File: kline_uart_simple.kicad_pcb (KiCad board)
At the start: 4 copper layers, 9 parts, among them J1 USB2UART, J2 KLINE_CONN, Q1 BC547, Q2 BC547

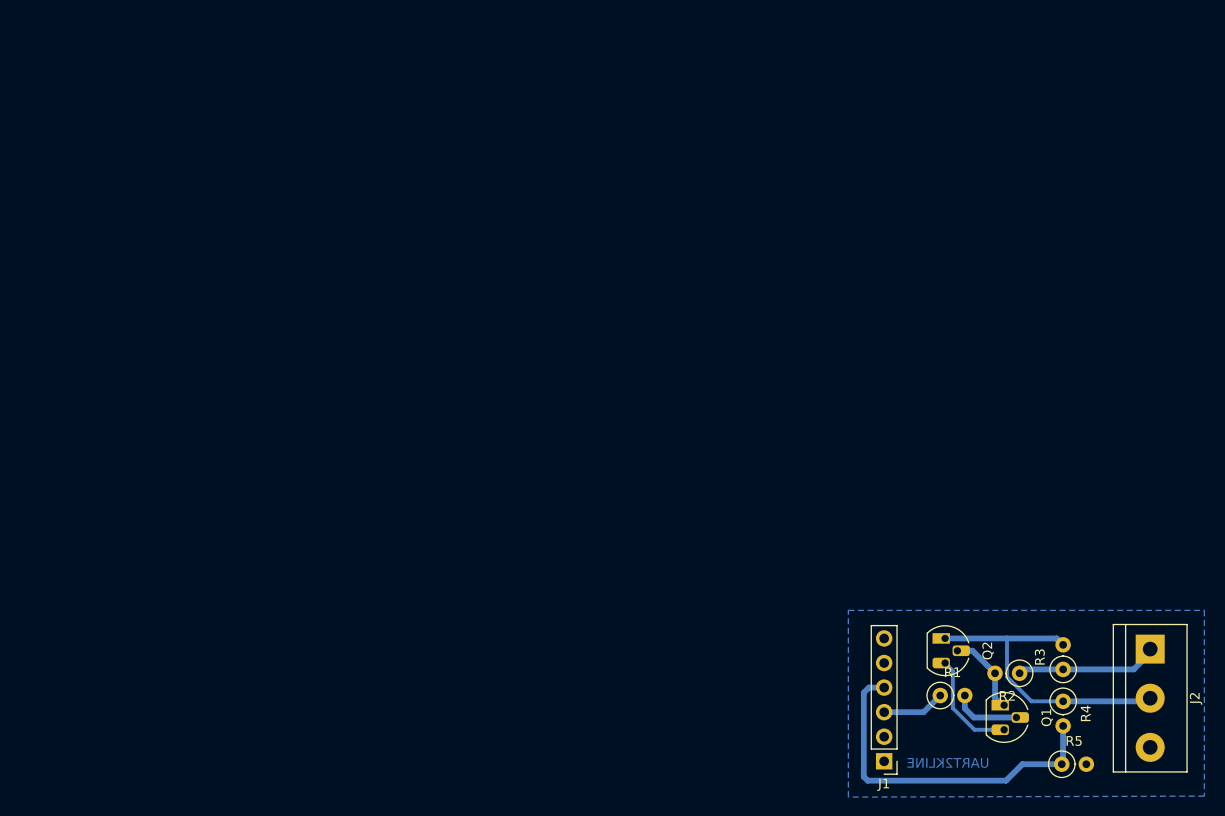
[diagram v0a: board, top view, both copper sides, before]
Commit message: new output pdf
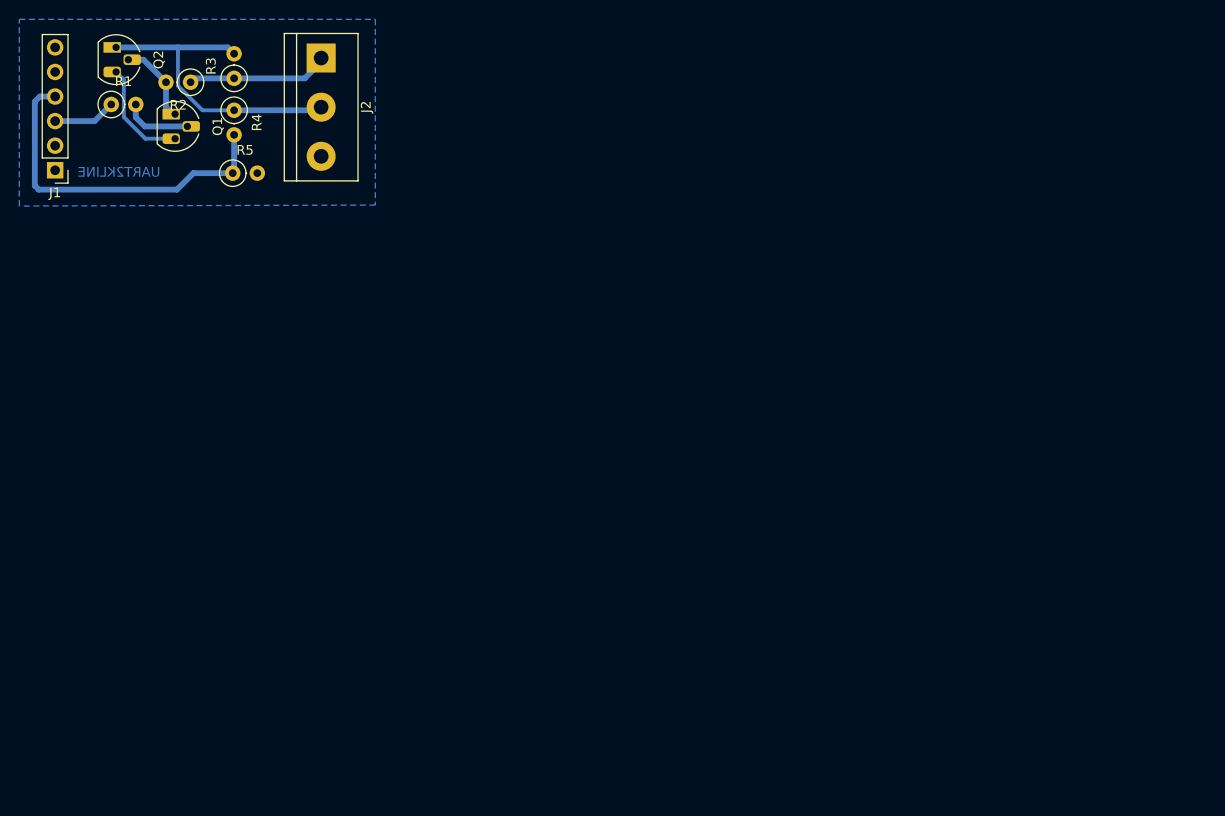
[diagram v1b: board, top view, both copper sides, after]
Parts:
- moved Q2 105.3 mm to (25.3, 19.8)
- moved R2 105.3 mm to (33.0, 23.4)
- moved R4 105.3 mm to (37.5, 26.3)
- moved R5 105.3 mm to (37.4, 32.8)
- moved J1 105.3 mm to (19.0, 32.5)
- moved J2 105.3 mm to (46.5, 20.9)
- moved Q1 105.3 mm to (31.4, 26.7)
- moved R1 105.3 mm to (24.8, 25.7)
- moved R3 105.3 mm to (37.5, 23.0)
